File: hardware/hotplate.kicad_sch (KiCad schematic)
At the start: 28 parts, among them J1 USB_C_Receptacle_USB2.0_16P, J2 Screw_Terminal_01x02, J3 Screw_Terminal_01x02, Q1 NMOS, SW1 SW_Push, U1 RP2040, U3 STUSB4500QTR, Y1 Crystal_GND24

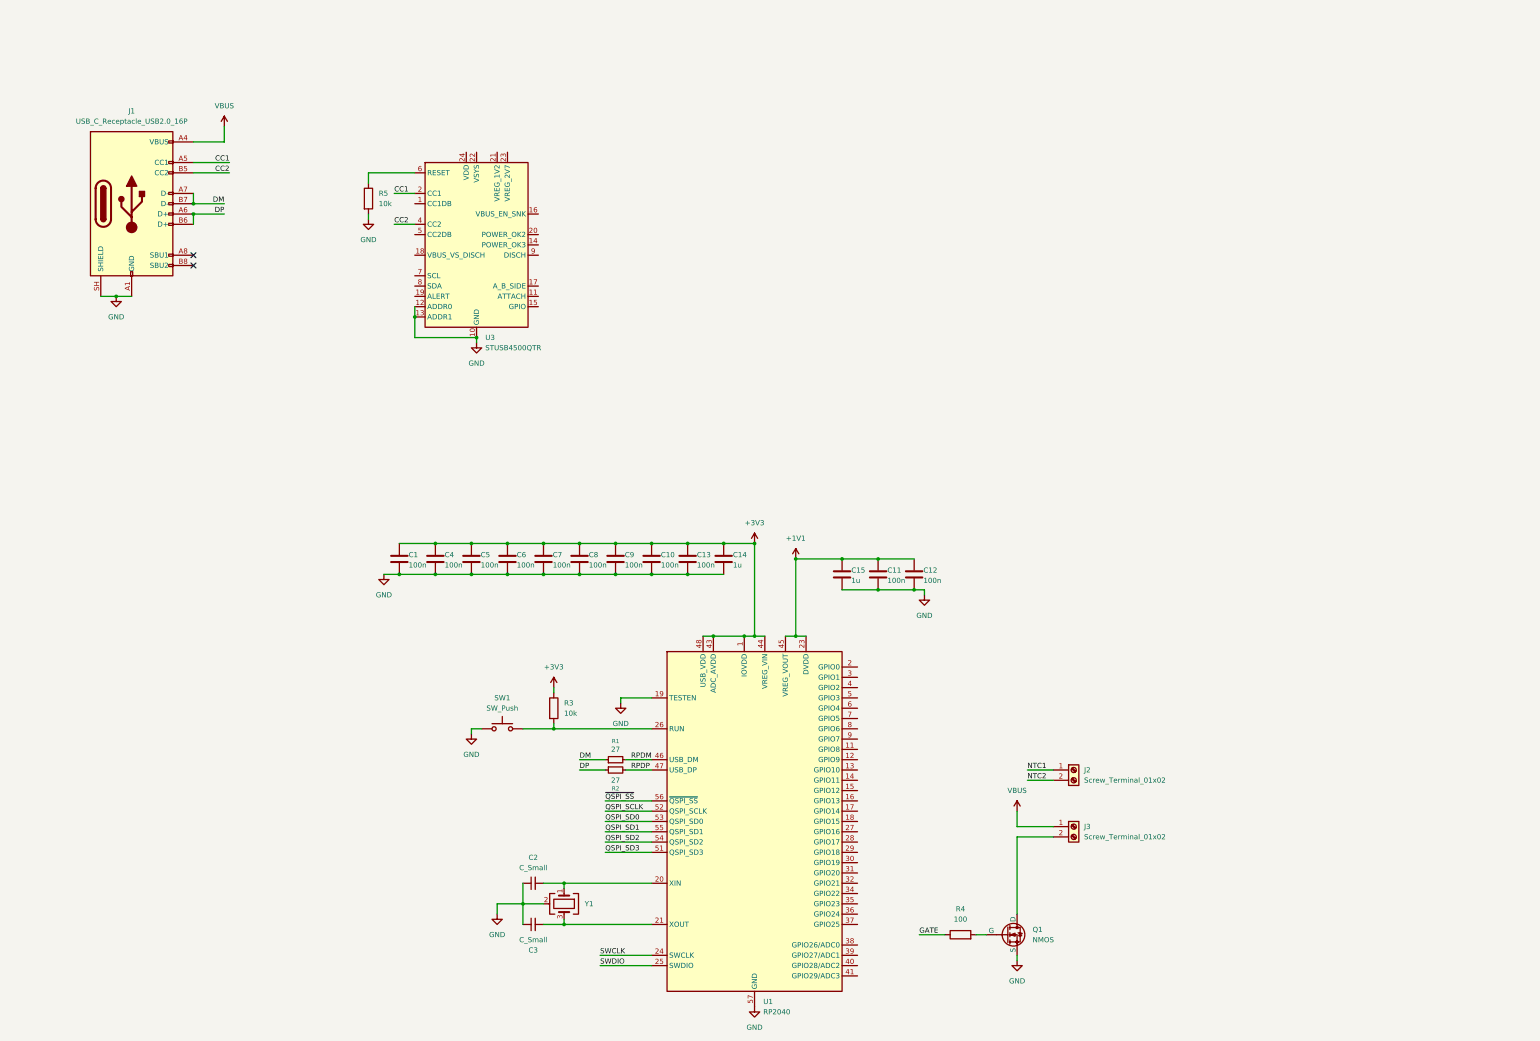
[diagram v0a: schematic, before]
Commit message: schematic complete(almost)
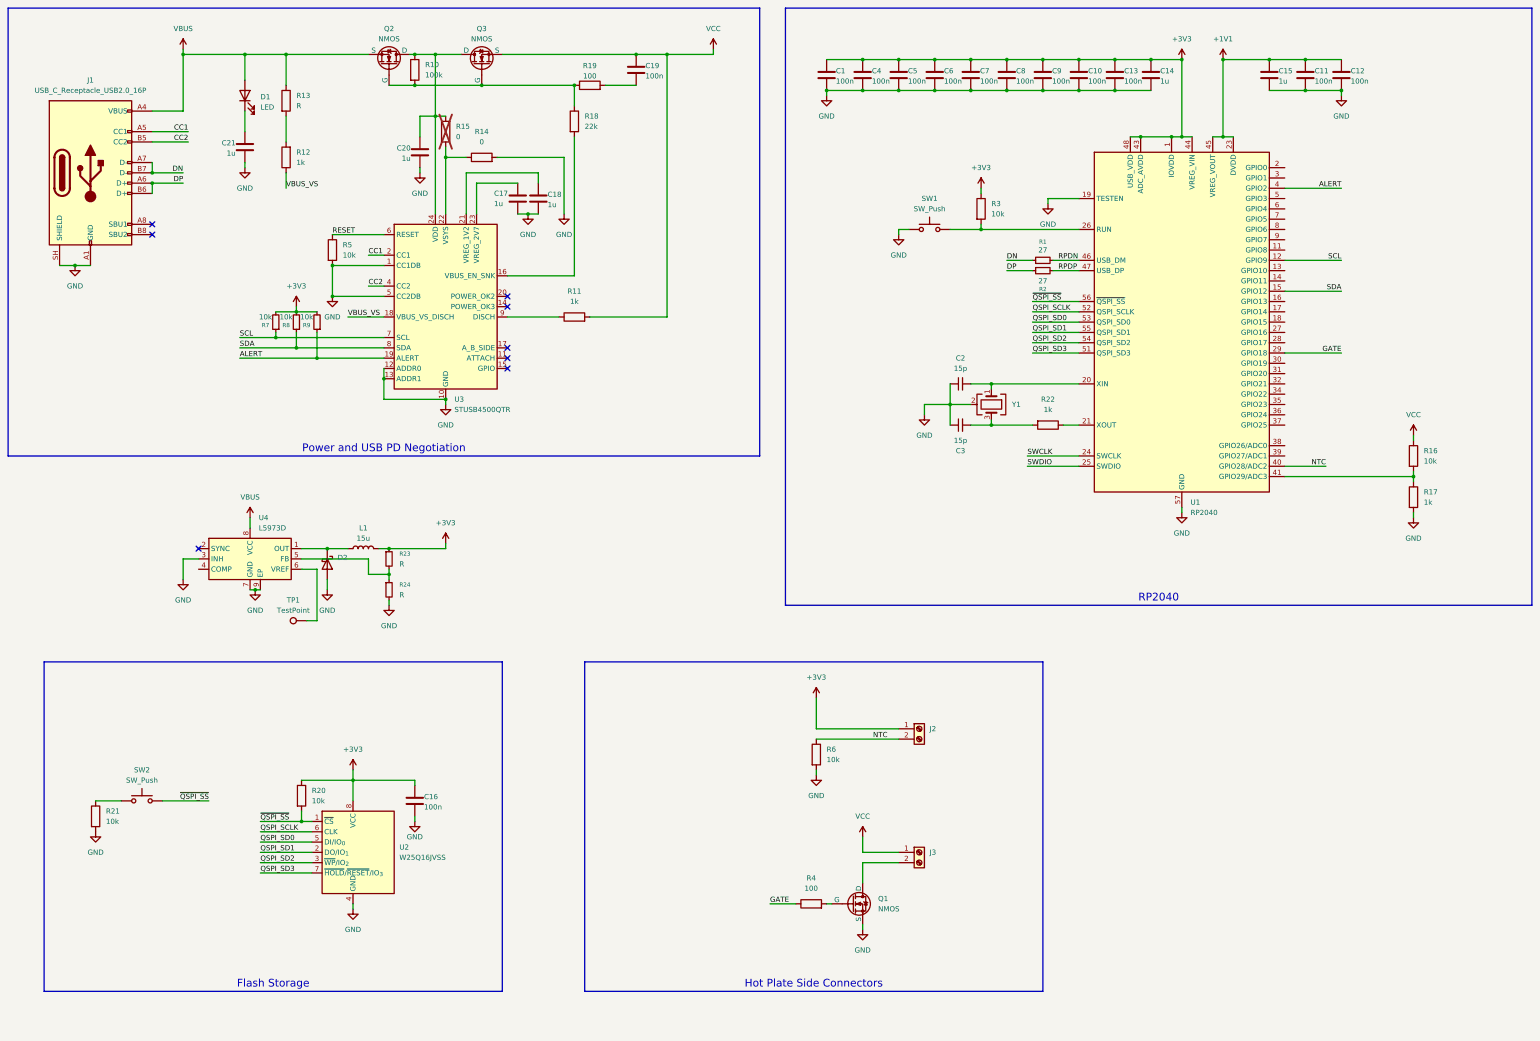
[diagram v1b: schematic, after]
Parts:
- added C16, C19: 100n, Capacitor_SMD:C_0402_1005Metric, symbol Device:C
- added C17, C18, C20, C21: 1u, Capacitor_SMD:C_0402_1005Metric, symbol Device:C
- added D1: LED, LED_SMD:LED_0402_1005Metric, symbol Device:LED
- added D2: D_Schottky, symbol Device:D_Schottky
- added L1: 15u, symbol Device:L
- added Q2, Q3: NMOS, symbol Simulation_SPICE:NMOS
- added R10: 100k, Resistor_SMD:R_0402_1005Metric, symbol Device:R
- added R11, R12, R17, R22: 1k, Resistor_SMD:R_0402_1005Metric, symbol Device:R
- added R13: R, Resistor_SMD:R_0402_1005Metric, symbol Device:R
- added R14, R15: 0, Resistor_SMD:R_0402_1005Metric, symbol Device:R
- added R16, R20, R21, R6: 10k, Resistor_SMD:R_0402_1005Metric, symbol Device:R
- added R18: 22k, Resistor_SMD:R_0402_1005Metric, symbol Device:R
- added R19: 100, Resistor_SMD:R_0402_1005Metric, symbol Device:R
- added R23, R24: R, symbol Device:R_Small
- added R7, R8, R9: 10k, Resistor_SMD:R_0402_1005Metric, symbol Device:R_Small
- added SW2: SW_Push, easyeda2kicad:SW-SMD_L3.9-W3.0-P4.45, symbol Switch:SW_Push
- added TP1: TestPoint, symbol Connector:TestPoint
- added U2: W25Q16JVSS, Package_SO:SOIC-8_5.3x5.3mm_P1.27mm, symbol Memory_Flash:W25Q16JVSS
- added U4: L5973D, Package_SO:HSOP-8-1EP_3.9x4.9mm_P1.27mm_EP2.41x3.1mm_ThermalVias, symbol Regulator_Switching:L5973D
- C2, C3: value C_Small -> 15p
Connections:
- net NTC1 is gone; now on net +3V3: J2.1 (Pin_1)
- net NTC2 is gone; now on net NTC: J2.2 (Pin_2)
- net +3V3: now also C16.1, L1.2, R20.1, R23.1, R7.2, R8.2, R9.2, U2.8 (VCC)
- net GATE: now also U1.29 (GPIO18)
- net GND: now also U3.1 (CC1DB), U3.5 (CC2DB), C16.2, C17.2, C18.2, C20.2, C21.2, D2.2 (A), R14.2, R17.2, R21.2, R24.2, R6.2, U2.4 (GND), U4.3 (INH), U4.7 (GND), U4.9 (EP)
- net QSPI_SCLK: now also U2.6 (CLK)
- net QSPI_SD0: now also U2.5 (DI/IO_{0})
- net QSPI_SD1: now also U2.2 (DO/IO_{1})
- net QSPI_SD2: now also U2.3 (~{WP}/IO_{2})
- net QSPI_SD3: now also U2.7 (~{HOLD}/~{RESET}/IO_{3})
- net VBUS: now also D1.2 (A), Q2.3 (S), R13.1, U4.8 (VCC); no longer J3.1 (Pin_1)
- net ~{QSPI_SS}: now also R20.2, SW2.2, U2.1 (~{CS})
- net at C3.2, Y1.3: now also R22.2; no longer U1.21 (XOUT)
- net RESET: now reaches R5.1, U3.6 (RESET)
- net SCL: now reaches U1.12 (GPIO9)
- net SCL: now also U3.7 (SCL), R7.1
- net SDA: now reaches U1.15 (GPIO12)
- net SDA: now also U3.8 (SDA), R8.1
- net ALERT: now reaches U1.4 (GPIO2)
- net ALERT: now also U3.19 (ALERT), R9.1
- net NTC: now reaches U1.40 (GPIO28/ADC2)
- net NTC: now also R6.1
- net at U1.41 (GPIO29/ADC3): now also R16.2, R17.1
- net at U3.16 (VBUS_EN_SNK): now also R18.2
- net VBUS_VS: now reaches U3.18 (VBUS_VS_DISCH)
- net VBUS_VS: now also R12.1
- net at U3.21 (VREG_1V2): now also C18.1
- net at U3.22 (VSYS): now also R14.1, R15.1
- net at U3.23 (VREG_2V7): now also C17.1
- net at U3.24 (VDD): now also C20.1, Q2.1 (D), Q3.1 (D), R10.1, R15.2
- net at U3.9 (DISCH): now also R11.1
- net DM renamed DN
- net RPDM renamed RPDN
- new net: R12.2, R13.2
- new net: R21.1, SW2.1
- new net: C21.1, D1.1 (K)
- new net: Q2.2 (G), Q3.2 (G), R10.2, R18.1, R19.1
- new net: D2.1 (K), L1.1, U4.1 (OUT)
- new net: R23.2, R24.1, U4.5 (FB)
- new net: TP1.1, U4.6 (VREF)
- new net: C19.2, R19.2
- new net: R22.1, U1.21 (XOUT)
- new net VCC: C19.1, J3.1 (Pin_1), Q3.3 (S), R11.2, R16.1
- no-connect marks 2 -> 8
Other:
- moved on the sheet: C1, C10, C11, C12, C13, C14, C15, C2, C3, C4, C5, C6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
